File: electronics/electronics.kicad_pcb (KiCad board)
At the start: 2 copper layers, 44.9 x 59.2 mm, 15 parts, among them J1 USB_C_Receptacle_USB2.0_14P, SW1 SW_Push, U1 ESP32-S3-WROOM-1, U3 NCP1117-3.3_SOT223, U5 NCP1117-3.3_SOT223

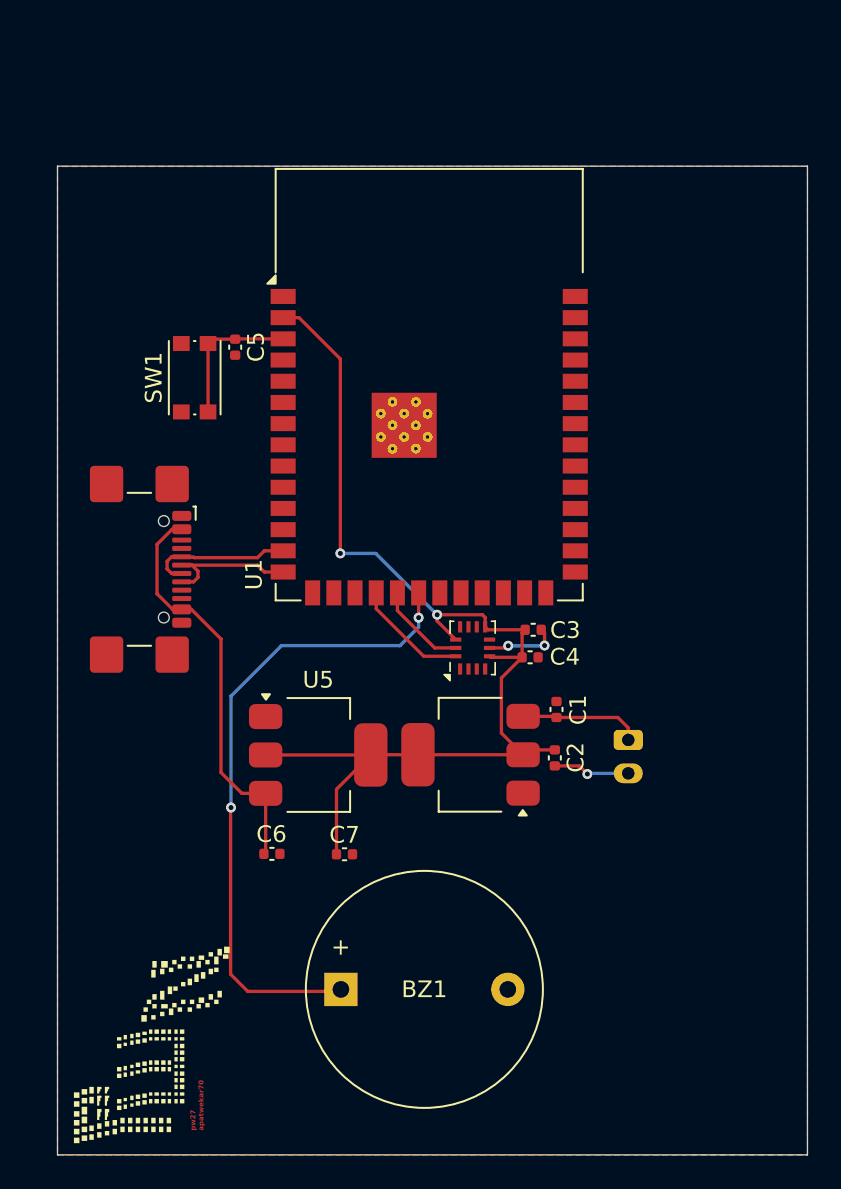
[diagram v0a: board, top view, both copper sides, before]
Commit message: PCB but better
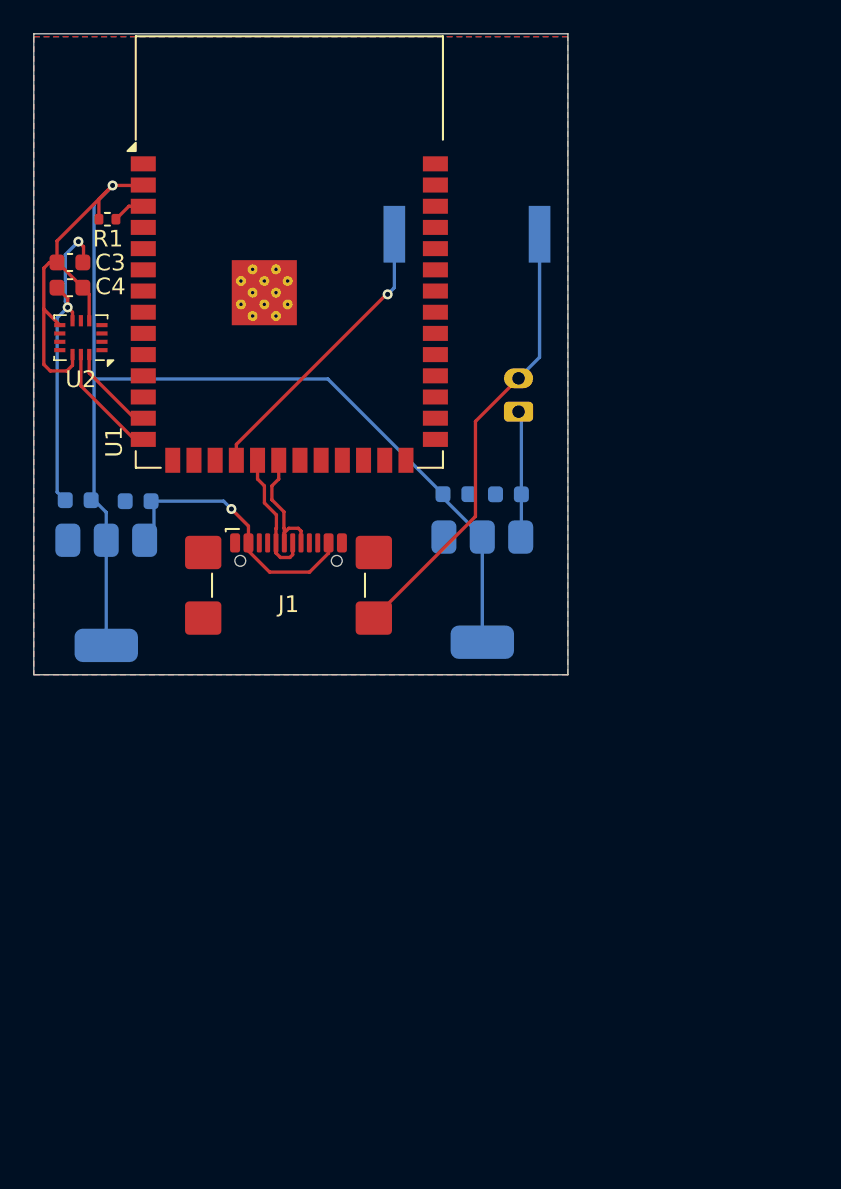
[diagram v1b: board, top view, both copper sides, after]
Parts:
- removed C5: 100nF, Capacitor_SMD:C_0402_1005Metric
- removed SW1: SW_Push, Button_Switch_SMD:SW_Push_1P1T_NO_CK_KMR2
- added R1: 10k, Resistor_SMD:R_0402_1005Metric, F.Cu at (132.1, 82.6)
- BZ1: footprint Buzzer_Beeper:Buzzer_D14mm_H7mm_P10mm -> Global:SPKR_PKMCS0909E4000-R1; moved to B.Cu
- C1, C2, C6, C7: footprint Capacitor_SMD:C_0402_1005Metric -> Capacitor_SMD:C_0603_1608Metric; moved to B.Cu
- C3, C4: footprint Capacitor_SMD:C_0402_1005Metric -> Capacitor_SMD:C_0603_1608Metric
- U3, U5: moved to B.Cu
- moved BZ1 45.9 mm to (153.7, 83.5)
- moved C3 35.4 mm to (129.9, 85.2)
- moved C4 35.4 mm to (129.9, 86.7), turned to 180 degrees
- moved U2 29.9 mm to (130.5, 89.7), turned to 180 degrees
- moved C7 26.5 mm to (130.4, 99.5), turned to 180 degrees
- moved C6 22.6 mm to (134.0, 99.5), turned to 180 degrees
- moved BT1 20.7 mm to (156.8, 94.2), turned to 90 degrees
- moved C2 16.9 mm to (153.0, 99.1), turned to 0 degrees
- moved U5 16.0 mm to (132.1, 105.0), turned to -90 degrees
- moved C1 13.2 mm to (156.1, 99.1), turned to 180 degrees
- moved U1 11.5 mm to (143.0, 84.6)
- moved J1 10.3 mm to (143.0, 105.7), turned to 0 degrees
- moved U3 9.92 mm to (154.6, 104.8), turned to -90 degrees
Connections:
- U1 pad 13: /D- -> /SDA
- U1 pad 14: /D+ -> /SCL
- U1 pad 18: /SDA -> /BZR
- U1 pad 19: /SCL -> /D-
- U1 pad 20: /BZR -> /D+
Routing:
- net GND: track 9.00 -> 47.4 mm, vias 3 -> 2
- net /BZR: track 38.7 -> 17.5 mm, vias 2 -> 1
- net +3V3: track 66.2 -> 87.2 mm, vias 2 -> 1
- net Net-(U5-VI): track 24.6 -> 16.7 mm, vias 0 -> 1
- net Net-(U1-EN): track 8.72 -> 1.96 mm
- net /SCL: track 5.48 -> 6.94 mm
- net /SDA: track 6.89 -> 5.47 mm
- net /D+: track 9.14 -> 7.92 mm
- net /D-: track 9.01 -> 7.92 mm
- added copper zone on B.Cu, net GND
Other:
- board size 44.9 x 59.2 mm -> 32 x 38.4 mm
- board text removed: "pw27 apatwekar70"
